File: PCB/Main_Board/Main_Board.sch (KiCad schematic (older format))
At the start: 11 parts, among them J1 USB_B_Micro, J2 Screw_Terminal_01x02, J3 SJ1-3523N, J4 SJ1-3523N, J5 Screw_Terminal_01x04, SW1 SW_SPDT, U1 TLV75533PDBV

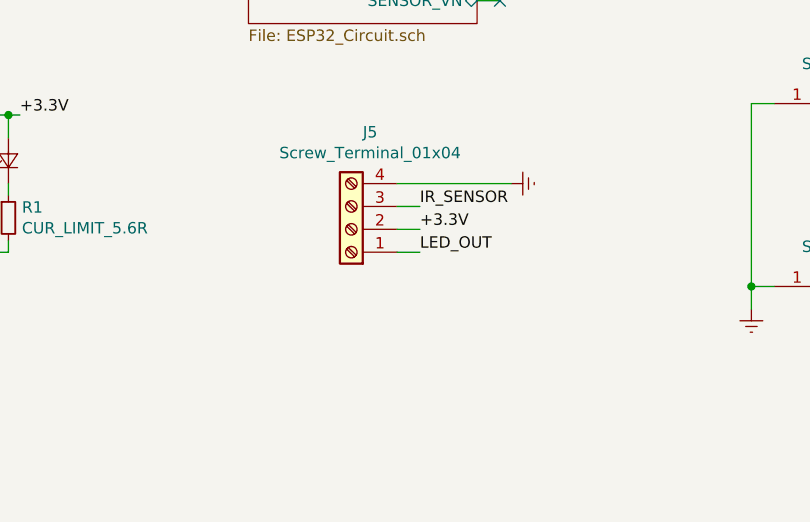
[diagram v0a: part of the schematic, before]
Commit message: PCB Layout work
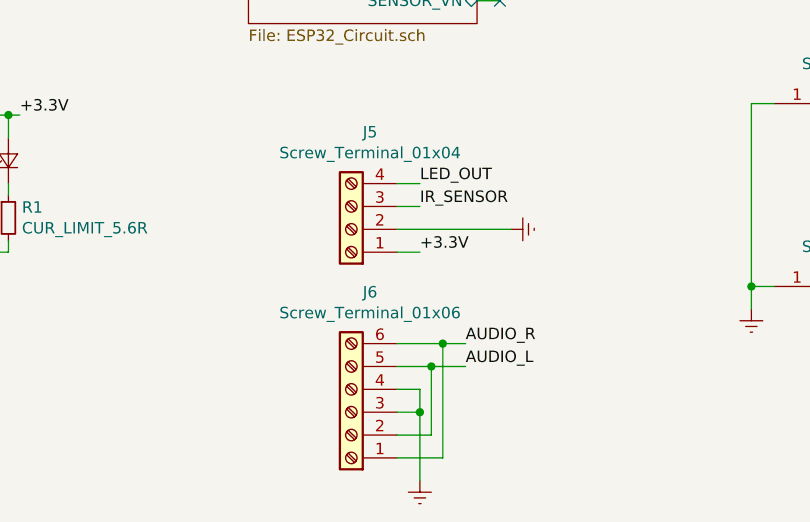
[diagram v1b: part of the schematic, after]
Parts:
- added J6: Screw_Terminal_01x06, TerminalBlock_Phoenix:TerminalBlock_Phoenix_MPT-0,5-6-2.54_1x06_P2.54mm_Horizontal, symbol Connector:Screw_Terminal_01x06
- J5: footprint TerminalBlock:TerminalBlock_bornier-4_P5.08mm -> TerminalBlock_Phoenix:TerminalBlock_Phoenix_MPT-0,5-4-2.54_1x04_P2.54mm_Horizontal
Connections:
- net +3.3V: now also J5.1 (Pin_1); no longer J5.2 (Pin_2)
- net AUDIO_L: now also J6.2 (Pin_2), J6.5 (Pin_5)
- net AUDIO_R: now also J6.1 (Pin_1), J6.6 (Pin_6)
- net Earth: now also J5.2 (Pin_2), J6.3 (Pin_3), J6.4 (Pin_4); no longer J5.4 (Pin_4)
- net LED_OUT: now also J5.4 (Pin_4); no longer J5.1 (Pin_1)
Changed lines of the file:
@@
 Text Label 6100 2400 2    50   ~ 0
 MSGEQ7_STROBE
-Text Label 4250 4650 0    50   ~ 0
+Text Label 4250 4350 0    50   ~ 0
 LED_OUT
 Text Label 4700 3050 0    50   ~ 0
@@
 Wire Wire Line
 	4500 1550 4700 1550
-$Comp
-L power:Earth #PWR05
-U 1 1 5F55AF8B
-P 4650 4350
-AR Path="/5F55AF8B" Ref="#PWR05"  Part="1"
-AR Path="/5F591C5D/5F55AF8B" Ref="#PWR?"  Part="1"
-F 0 "#PWR05" H 4650 4100 50  0001 C CNN
-F 1 "Earth" H 4650 4200 50  0001 C CNN
-F 2 "" H 4650 4350 50  0001 C CNN
-F 3 "~" H 4650 4350 50  0001 C CNN
-	1    4650 4350
-	0    -1   -1   0
-$EndComp
-Text Label 4250 4550 0    50   ~ 0
-+3.3V
 Text Label 4700 2950 0    50   ~ 0
 IR_SENSOR
 Wire Wire Line
 	4500 2950 4700 2950
-Text Label 4250 4450 0    50   ~ 0
-IR_SENSOR
 $Comp
 L SamacSys:SJ1-3523N J3
@@
 F 0 "J5" H 3868 4125 50  0000 C CNN
 F 1 "Screw_Terminal_01x04" H 3868 4216 50  0000 C CNN
-F 2 "TerminalBlock:TerminalBlock_bornier-4_P5.08mm" H 3950 4550 50  0001 C CNN
+F 2 "TerminalBlock_Phoenix:TerminalBlock_Phoenix_MPT-0,5-4-2.54_1x04_P2.54mm_Horizontal" H 3950 4550 50  0001 C CNN
 F 3 "~" H 3950 4550 50  0001 C CNN
 F 4 "https://www.mouser.co.uk/ProductDetail/CUI-Devices/TB006-508-04BE?qs=vLWxofP3U2zpUvBkDCHiCA%3D%3D" H 3950 4550 50  0001 C CNN "Product"
@@
 $EndComp
 Wire Wire Line
-	4150 4350 4650 4350
-Wire Wire Line
 	4150 4450 4250 4450
 Wire Wire Line
-	4150 4550 4250 4550
-Wire Wire Line
 	4150 4650 4250 4650
 Wire Wire Line
+	4150 4350 4250 4350
+Wire Wire Line
 	1450 1900 1750 1900
 Wire Wire Line
@@
 Wire Wire Line
 	1150 2550 1150 2700
+$Comp
+L Connector:Screw_Terminal_01x06 J6
+U 1 1 5F57EA02
+P 3950 5350
+F 0 "J6" H 3868 4825 50  0000 C CNN
+F 1 "Screw_Terminal_01x06" H 3868 4916 50  0000 C CNN
+F 2 "TerminalBlock_Phoenix:TerminalBlock_Phoenix_MPT-0,5-6-2.54_1x06_P2.54mm_Horizontal" H 3950 5350 50  0001 C CNN
+F 3 "~" H 3950 5350 50  0001 C CNN
+	1    3950 5350
+	-1   0    0    1
+$EndComp
+Wire Wire Line
+	4150 5250 4250 5250
+Wire Wire Line
+	4250 5250 4250 5350
+Wire Wire Line
+	4250 5350 4150 5350
+$Comp
+L power:Earth #PWR0101
+U 1 1 5F590EF5
+P 4250 5650
+AR Path="/5F590EF5" Ref="#PWR0101"  Part="1"
+AR Path="/5F591C5D/5F590EF5" Ref="#PWR?"  Part="1"
+F 0 "#PWR0101" H 4250 5400 50  0001 C CNN
+F 1 "Earth" H 4250 5500 50  0001 C CNN
+F 2 "" H 4250 5650 50  0001 C CNN
+F 3 "~" H 4250 5650 50  0001 C CNN
+	1    4250 5650
+	1    0    0    -1
+$EndComp
+Connection ~ 4250 5350
+Text Label 4450 5150 0    50   ~ 0
+AUDIO_L
+Wire Wire Line
+	4250 5350 4250 5650
+Wire Wire Line
+	4150 5150 4300 5150
+Wire Wire Line
+	4150 5450 4300 5450
+Wire Wire Line
+	4300 5450 4300 5150
+Wire Wire Line
+	4150 5050 4350 5050
+Wire Wire Line
+	4350 5050 4350 5550
+Wire Wire Line
+	4350 5550 4150 5550
+Text Label 4450 5050 0    50   ~ 0
+AUDIO_R
+Wire Wire Line
+	4450 5050 4350 5050
+Connection ~ 4350 5050
+Wire Wire Line
+	4450 5150 4300 5150
+Connection ~ 4300 5150
+Text Label 4250 4450 0    50   ~ 0
+IR_SENSOR
+$Comp
+L power:Earth #PWR05
+U 1 1 5F55AF8B
+P 4650 4550
+AR Path="/5F55AF8B" Ref="#PWR05"  Part="1"
+AR Path="/5F591C5D/5F55AF8B" Ref="#PWR?"  Part="1"
+F 0 "#PWR05" H 4650 4300 50  0001 C CNN
+F 1 "Earth" H 4650 4400 50  0001 C CNN
+F 2 "" H 4650 4550 50  0001 C CNN
+F 3 "~" H 4650 4550 50  0001 C CNN
+	1    4650 4550
+	0    -1   -1   0
+$EndComp
+Text Label 4250 4650 0    50   ~ 0
++3.3V
+Wire Wire Line
+	4150 4550 4650 4550
 $EndSCHEMATC
